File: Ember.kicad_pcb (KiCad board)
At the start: 2 copper layers, 2 parts, among them J1 FT232H Left, J2 FT232H Right

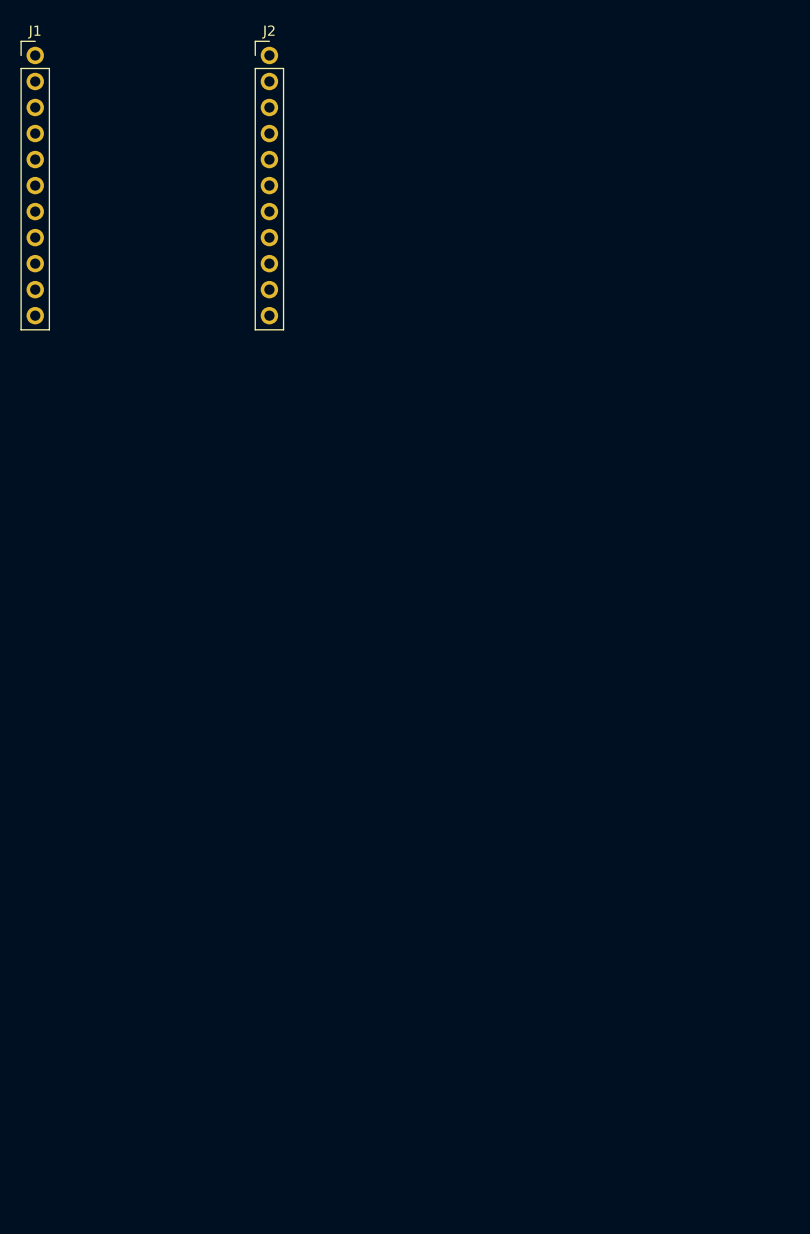
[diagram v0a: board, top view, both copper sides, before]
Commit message: Built the whole v1.0 design in one day
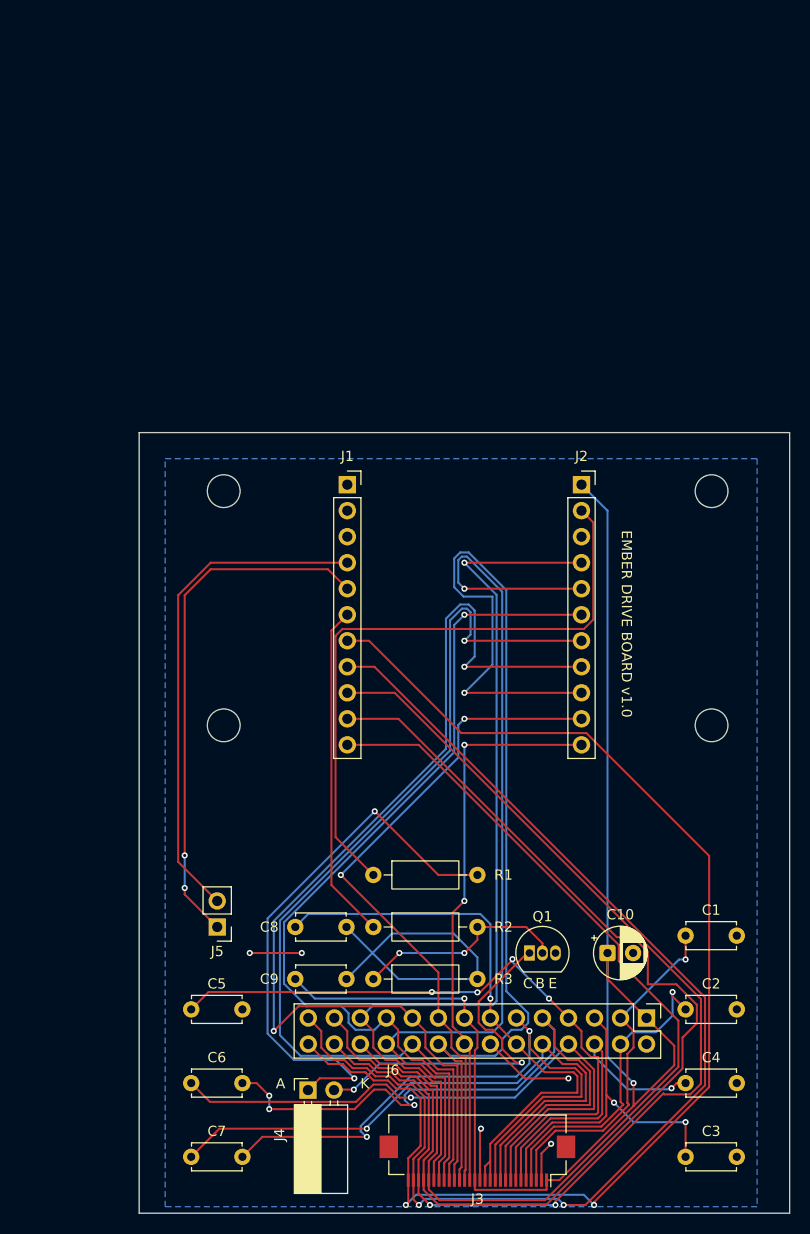
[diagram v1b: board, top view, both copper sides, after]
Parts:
- added C1: 1uF, Capacitor_THT:C_Disc_D4.7mm_W2.5mm_P5.00mm, F.Cu at (170.0, 111.1)
- added C10: 10uF, Capacitor_THT:CP_Radial_D5.0mm_P2.50mm, F.Cu at (162.4, 112.8)
- added C2: 1uF, Capacitor_THT:C_Disc_D4.7mm_W2.5mm_P5.00mm, F.Cu at (170.0, 118.3)
- added C3: 1uF, Capacitor_THT:C_Disc_D4.7mm_W2.5mm_P5.00mm, F.Cu at (170.0, 132.7)
- added C4: 1uF, Capacitor_THT:C_Disc_D4.7mm_W2.5mm_P5.00mm, F.Cu at (170.0, 125.5)
- added C5: 1uF, Capacitor_THT:C_Disc_D4.7mm_W2.5mm_P5.00mm, F.Cu at (121.7, 118.3)
- added C6: 1uF, Capacitor_THT:C_Disc_D4.7mm_W2.5mm_P5.00mm, F.Cu at (121.7, 125.5)
- added C7: 1uF, Capacitor_THT:C_Disc_D4.7mm_W2.5mm_P5.00mm, F.Cu at (121.7, 132.7)
- added C8: 1uF, Capacitor_THT:C_Disc_D4.7mm_W2.5mm_P5.00mm, F.Cu at (131.9, 110.3)
- added C9: 100nF, Capacitor_THT:C_Disc_D4.7mm_W2.5mm_P5.00mm, F.Cu at (131.9, 115.3)
- added J3: LCD Panel - 28 Pin Tail, Connector_FFC-FPC:Hirose_FH12-28S-0.5SH_1x28-1MP_P0.50mm_Horizontal, F.Cu at (149.7, 133.1)
- added J4: LCD Backlight, Connector_PinSocket_2.54mm:PinSocket_1x02_P2.54mm_Horizontal, F.Cu at (133.1, 126.2)
- added J5: Spare GPIO, Connector_PinHeader_2.54mm:PinHeader_1x02_P2.54mm_Vertical, F.Cu at (124.3, 110.3)
- added J6: Debug Pads, Connector_PinHeader_2.54mm:PinHeader_2x14_P2.54mm_Vertical, F.Cu at (166.2, 119.1)
- added Q1: P2N2222A, Package_TO_SOT_THT:TO-92_Inline, F.Cu at (154.8, 112.8)
- added R1: 220, Resistor_THT:R_Axial_DIN0207_L6.3mm_D2.5mm_P10.16mm_Horizontal, F.Cu at (139.5, 105.2)
- added R2: 1k, Resistor_THT:R_Axial_DIN0207_L6.3mm_D2.5mm_P10.16mm_Horizontal, F.Cu at (139.5, 110.3)
- added R3: 10k, Resistor_THT:R_Axial_DIN0207_L6.3mm_D2.5mm_P10.16mm_Horizontal, F.Cu at (139.5, 115.3)
- added REF**: MountingHole_3.2mm_M3, MountingHole:MountingHole_3.2mm_M3, F.Cu at (172.5, 90.6)
- added REF**: MountingHole_3.2mm_M3, MountingHole:MountingHole_3.2mm_M3, F.Cu at (124.9, 67.7)
- added REF**: MountingHole_3.2mm_M3, MountingHole:MountingHole_3.2mm_M3, F.Cu at (172.5, 67.7)
- added REF**: MountingHole_3.2mm_M3, MountingHole:MountingHole_3.2mm_M3, F.Cu at (124.9, 90.6)
- J1: value FT232H Left -> FT232H Control; footprint Connector_PinHeader_2.54mm:PinHeader_1x11_P2.54mm_Vertical -> Connector_PinSocket_2.54mm:PinSocket_1x11_P2.54mm_Vertical
- J2: value FT232H Right -> FT232H Power + Data; footprint Connector_PinHeader_2.54mm:PinHeader_1x11_P2.54mm_Vertical -> Connector_PinSocket_2.54mm:PinSocket_1x11_P2.54mm_Vertical
- moved J1 51.8 mm to (137.0, 67.1)
- moved J2 51.8 mm to (159.8, 67.1)
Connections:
- J1 pad 1: unconnected-(J1-Pin_1-Pad1) -> GND
- J1 pad 10: unconnected-(J1-Pin_10-Pad10) -> /C1
- J1 pad 11: unconnected-(J1-Pin_11-Pad11) -> /C0
- J1 pad 4: unconnected-(J1-Pin_4-Pad4) -> /C7
- J1 pad 5: unconnected-(J1-Pin_5-Pad5) -> /C6
- J1 pad 6: unconnected-(J1-Pin_6-Pad6) -> /C5
- J1 pad 7: unconnected-(J1-Pin_7-Pad7) -> /C4
- J1 pad 8: unconnected-(J1-Pin_8-Pad8) -> /C3
- J1 pad 9: unconnected-(J1-Pin_9-Pad9) -> /C2
- J2 pad 1: unconnected-(J2-Pin_1-Pad1) -> +3V3
- J2 pad 10: unconnected-(J2-Pin_10-Pad10) -> /D6
- J2 pad 11: unconnected-(J2-Pin_11-Pad11) -> /D7
- J2 pad 2: unconnected-(J2-Pin_2-Pad2) -> +5V
- J2 pad 3: unconnected-(J2-Pin_3-Pad3) -> GND
- J2 pad 4: unconnected-(J2-Pin_4-Pad4) -> /D0
- J2 pad 5: unconnected-(J2-Pin_5-Pad5) -> /D1
- J2 pad 6: unconnected-(J2-Pin_6-Pad6) -> /D2
- J2 pad 7: unconnected-(J2-Pin_7-Pad7) -> /D3
- J2 pad 8: unconnected-(J2-Pin_8-Pad8) -> /D4
- J2 pad 9: unconnected-(J2-Pin_9-Pad9) -> /D5
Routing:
- net +3V3: track 0.00 -> 138.0 mm, vias 0 -> 2
- net /C4: track 0.00 -> 126.1 mm, vias 0 -> 2
- net /C3: track 0.00 -> 116.9 mm, vias 0 -> 2
- net /C2: track 0.00 -> 109.8 mm, vias 0 -> 2
- net /C1: track 0.00 -> 109.3 mm
- net /D5: track 0.00 -> 104.7 mm, vias 0 -> 1
- net /D4: track 0.00 -> 101.8 mm, vias 0 -> 2
- net /C0: track 0.00 -> 98.7 mm
- net /D3: track 0.00 -> 94.7 mm, vias 0 -> 1
- net /D1: track 0.00 -> 91.9 mm, vias 0 -> 1
- net /D0: track 0.00 -> 90.8 mm, vias 0 -> 1
- net /D2: track 0.00 -> 87.6 mm, vias 0 -> 1
- net /D6: track 0.00 -> 66.8 mm, vias 0 -> 2
- net /PUMP_9: track 0.00 -> 66.0 mm, vias 0 -> 3
- net /BIAS7: track 0.00 -> 65.0 mm, vias 0 -> 4
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- added copper zone on B.Cu, net GND
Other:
- board outline added: 63.5 x 76.2 mm
- board text added: "A"
- board text added: "B"
- board text added: "C"
- board text added: "E"
- board text added: "EMBER DRIVE BOARD v1.0"
- board text added: "K"
